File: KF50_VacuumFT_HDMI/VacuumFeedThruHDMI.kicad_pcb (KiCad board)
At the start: 4 copper layers, 142 x 154 mm, 16 parts, among them J1 - (5:8) HDMI_A_1.4, J1 - (9:12) HDMI_A_1.4, J1 DB25_Male, J1- (1:4) HDMI_A_1.4, J2 - (1:4) HDMI_A_1.4, J2 - (5:8) HDMI_A_1.4, J2 - (9:12) HDMI_A_1.4, J2 Conn_01x08, J2 DB25_Male, J3 - (1:4) HDMI_A_1.4, J3 - (5:8) HDMI_A_1.4, J3 - (9:12) HDMI_A_1.4, J3 DB25_Male

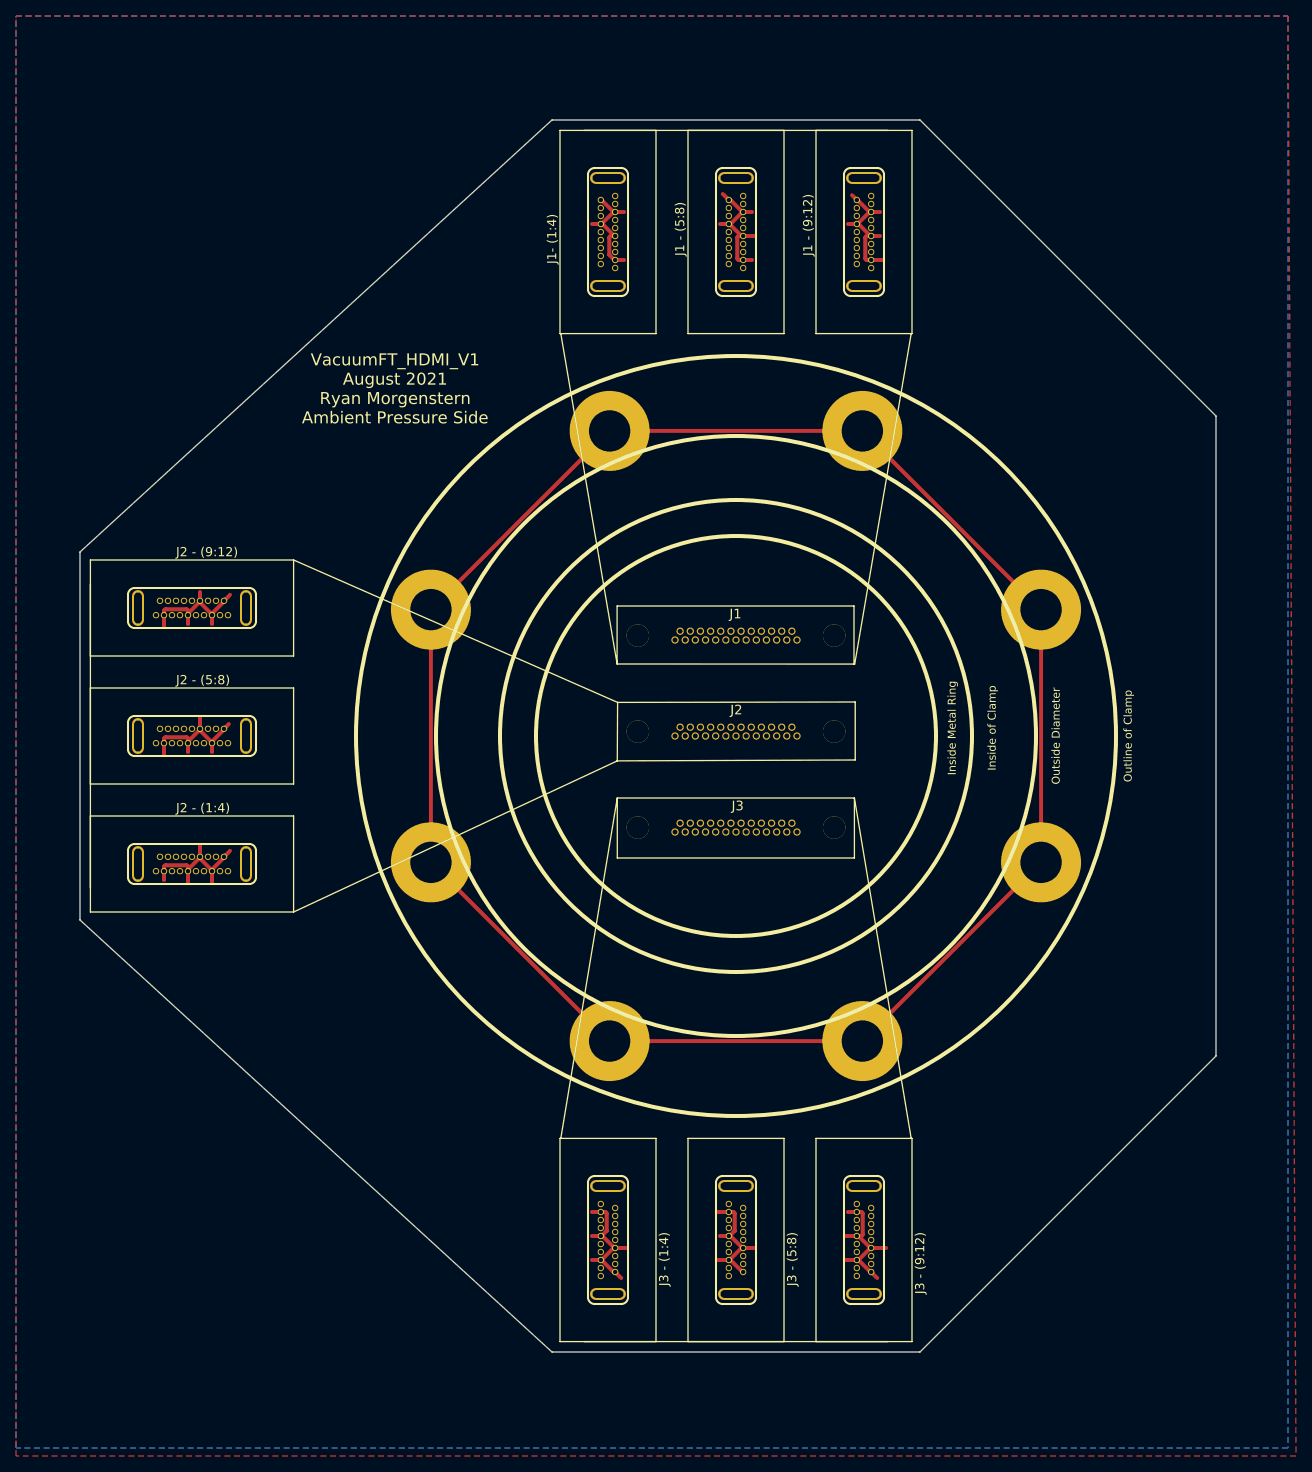
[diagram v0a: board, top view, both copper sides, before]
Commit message: Updated Gerber
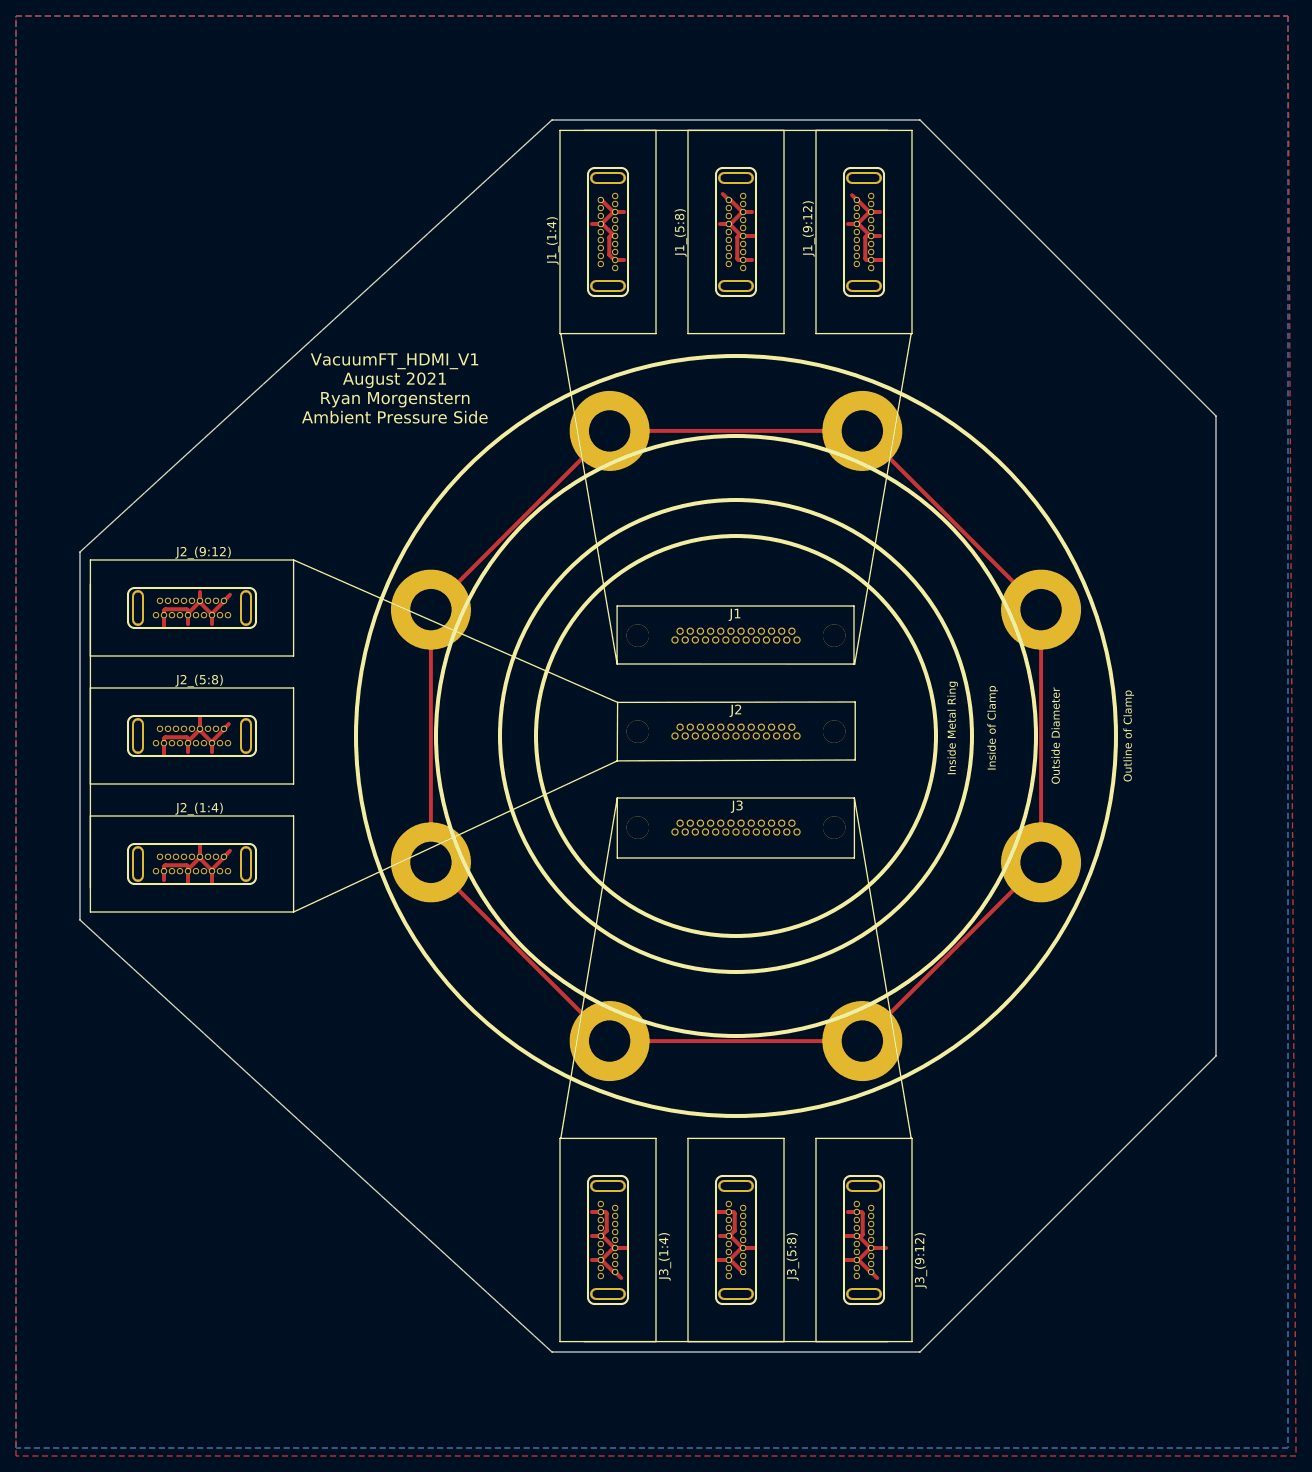
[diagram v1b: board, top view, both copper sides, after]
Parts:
- J1_(1:4): renamed from J1- (1:4)
- J1_(5:8): renamed from J1 - (5:8)
- J1_(9:12): renamed from J1 - (9:12)
- J2_(1:4): renamed from J2 - (1:4)
- J2_(5:8): renamed from J2 - (5:8)
- J2_(9:12): renamed from J2 - (9:12)
- J3_(1:4): renamed from J3 - (1:4)
- J3_(5:8): renamed from J3 - (5:8)
- J3_(9:12): renamed from J3 - (9:12)
